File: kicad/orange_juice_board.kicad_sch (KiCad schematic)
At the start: 54 parts, among them J10 PWM_OUT1, J11 CONN_UART, J12 PWM_OUT2, J13 FAN_12/24v, J15 PWM_OUT3, J2 DC_INPUT, J3 CONN_ADXL345, J4 OrangePi Zero GPIO PINs, J5 Conn_MAX31865, J7 OrangePi Zero Function Interf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, J8 FAN_5v, J9 PWR_5v, Q1 AO3401A, Q2 AO3400A, Q3 AO3400A, Q4 AO3400A, U1 TPS5430

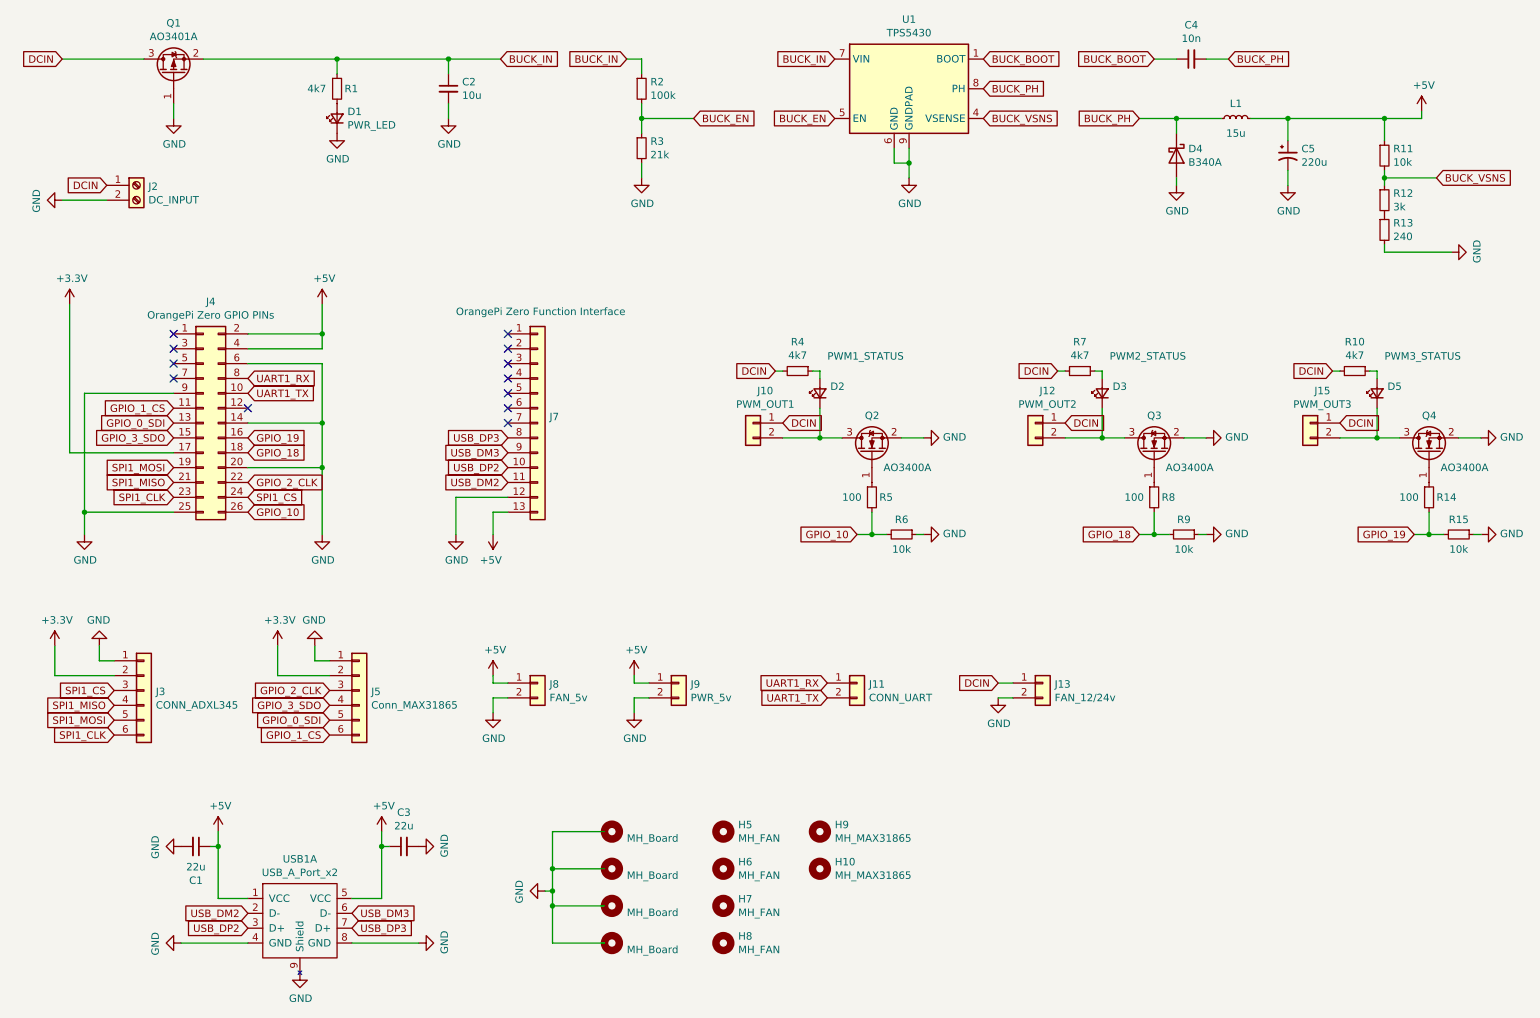
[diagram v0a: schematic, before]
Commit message: update version 0.3
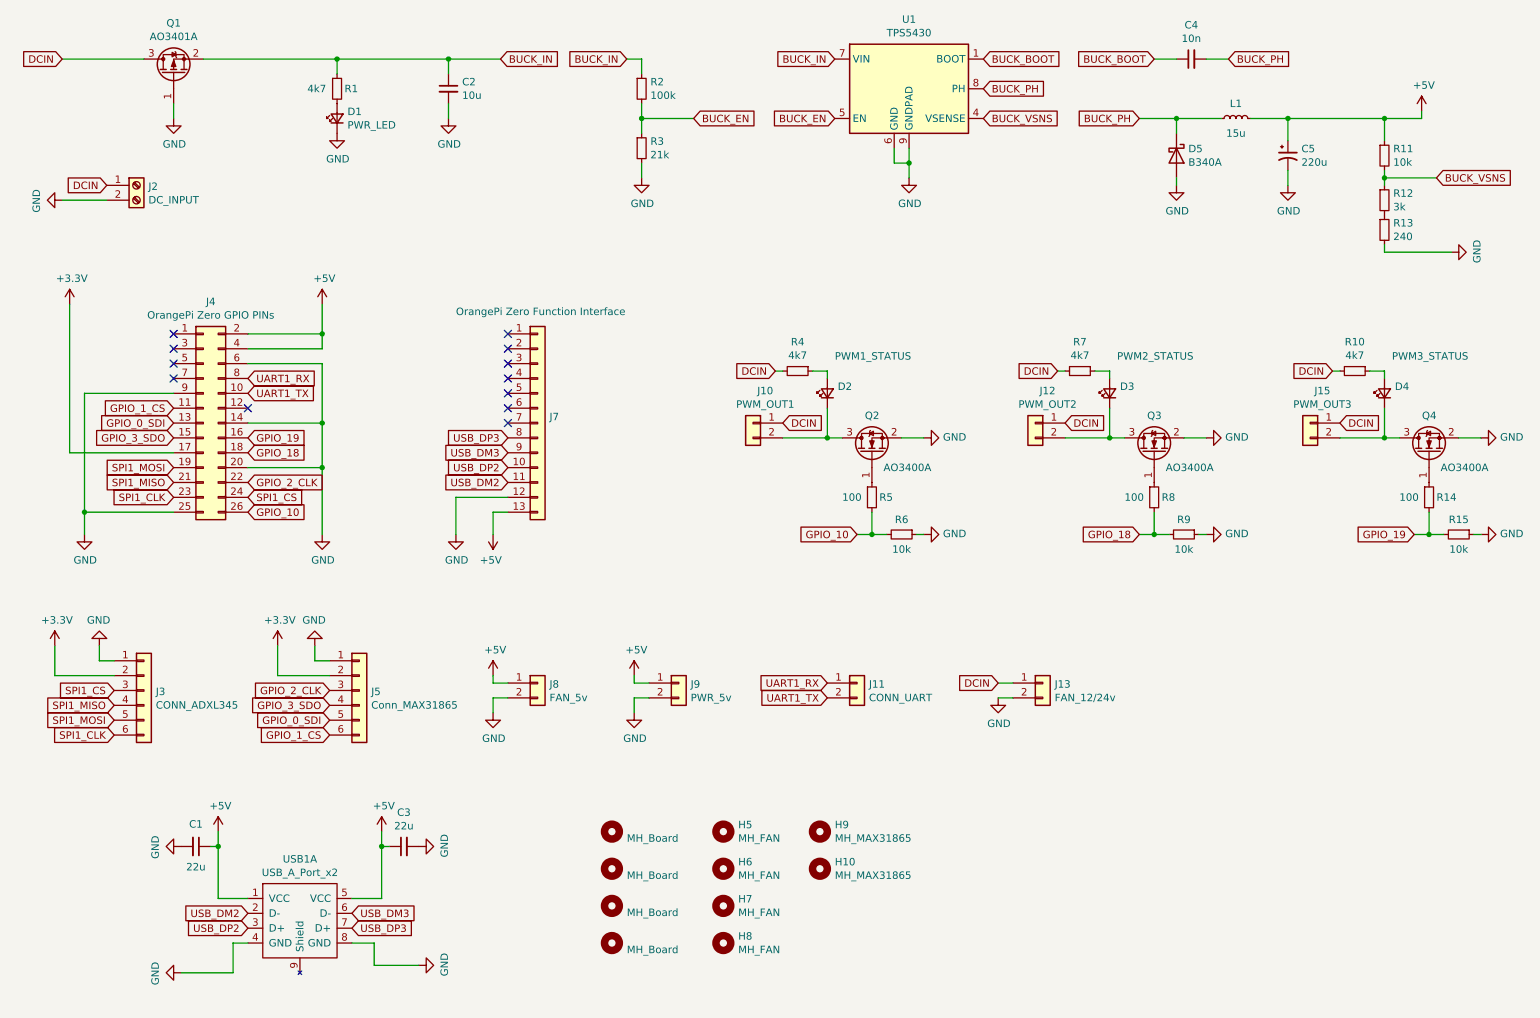
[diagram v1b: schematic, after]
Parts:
- renumbered D5 to D4, D4 to D5
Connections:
- net GND: no longer USB1.9 (Shield)
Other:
- moved on the sheet: D2, D3, D4
